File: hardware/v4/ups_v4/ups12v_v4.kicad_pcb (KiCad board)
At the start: 4 copper layers, 152 parts, among them IC1 BQ25798RQMR, J1 ADAPTER 4.75-21V, J2 VSYS OUTPUT, J3 BATTERY 2S/4S, J4 MCU / BIAS INTERFACE, J6 NTC temp sensor, J7 USB-C PROGRAM / NATIVE USB, J8 5V / GND, Q1 AON7528, Q10 AON7528, Q2 AON7528, Q3 PMV16UN, Q4 BC847 INT DOMAIN ISOLATOR, Q5 BC857 MAIN-GATED CHG SOURCE, Q6 BC847 MAIN_VALID SINK, Q7 BC847 MCU CHG ARM SINK, Q8 PMV16UN MAIN_VALID, Q9 PMV16UN TCA_EN, SW1 BOOT / DOWNLOAD, SW2 RESET, U1 ESP32-C3-MINI-1-N4X, U2 TPD2EUSB30A (PROVISIONAL), U3 TPS62933DRLR NORMAL 3V3, U4 AP7361C-33E-13 USB 3V3 LDO, U5 TPS2116DRL NORMAL PRIORITY, U6 TCA9517DGKR REV.D, U7 TPS62933DRLR, U8 LM74700QDBVRQ1

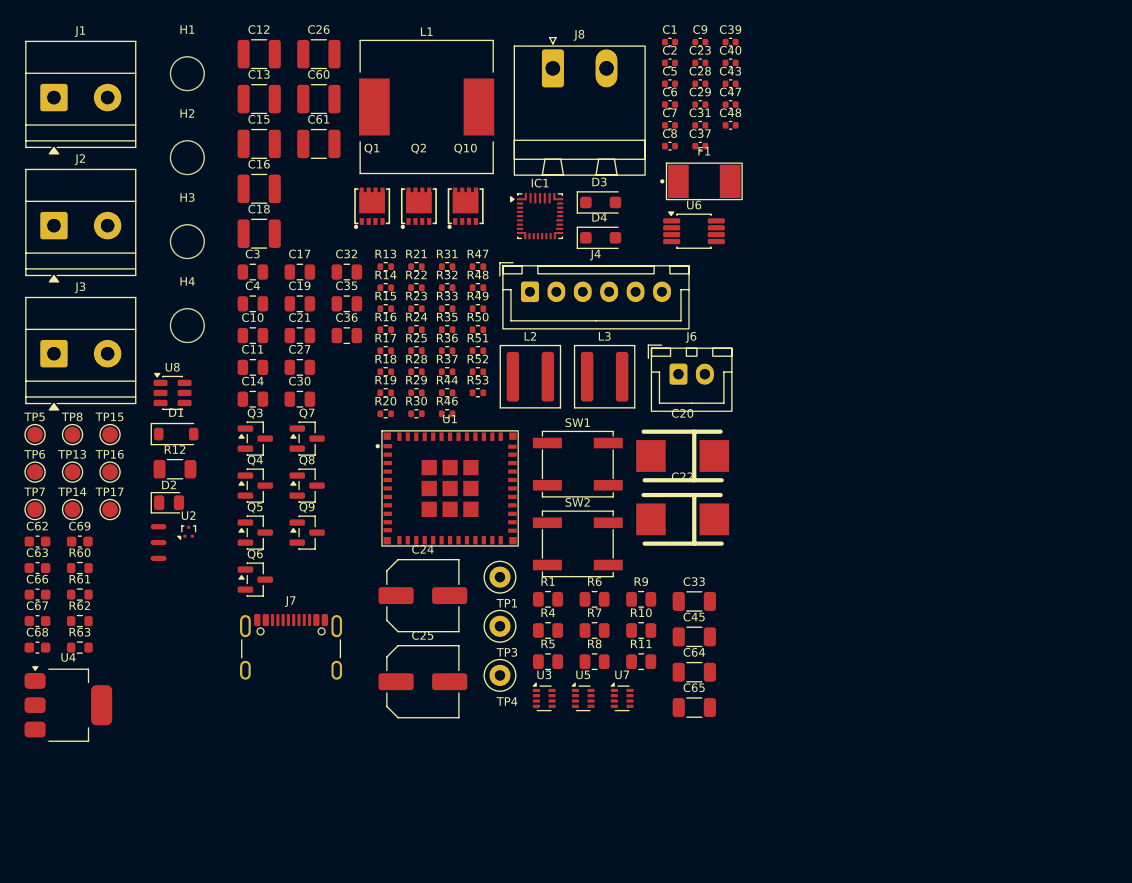
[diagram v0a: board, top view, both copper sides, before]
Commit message: phase 4.3
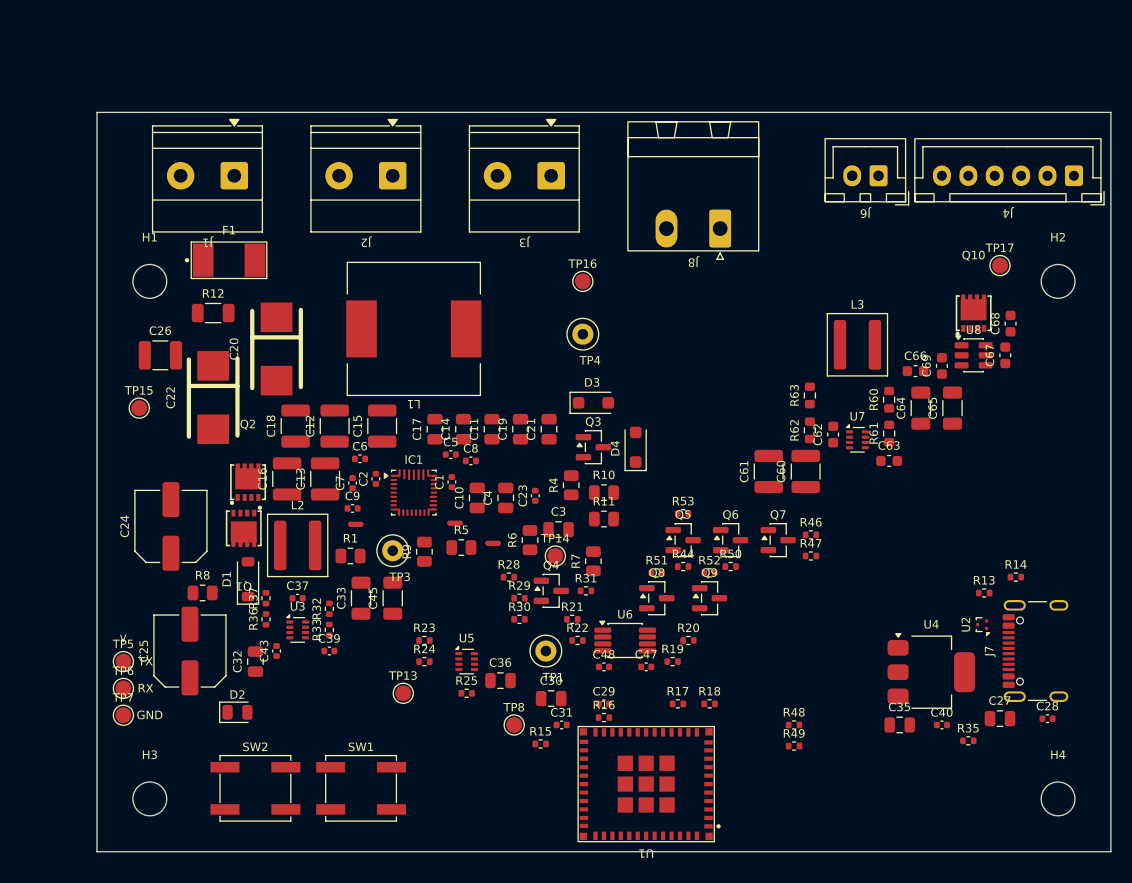
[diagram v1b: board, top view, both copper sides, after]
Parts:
- moved C68 97.1 mm to (116.5, 50.0), turned to 90 degrees
- moved C67 95.0 mm to (116.0, 53.0), turned to 90 degrees
- moved H4 93.8 mm to (121.0, 95.0)
- moved TP17 87.4 mm to (115.5, 44.5)
- moved C66 85.8 mm to (107.5, 54.5)
- moved C69 83.3 mm to (110.0, 54.0), turned to 90 degrees
- moved H2 83.3 mm to (121.0, 46.0)
- moved U4 81.8 mm to (109.0, 83.0)
- moved C63 81.3 mm to (105.0, 63.0)
- moved R60 78.3 mm to (105.0, 57.2), turned to 90 degrees
- moved R61 78.1 mm to (105.0, 60.4), turned to 90 degrees
- moved C62 76.0 mm to (99.7, 60.5), turned to 90 degrees
- moved U8 75.9 mm to (113.0, 53.0)
- moved U2 75.6 mm to (113.8, 78.5), turned to 90 degrees
- moved C27 74.2 mm to (115.5, 87.4)
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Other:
- board outline added: 96 x 70 mm
- board text added: ">"
- board text added: "GND"
- board text added: "RF: ALL LAYERS CLEAR - 15 mm EXTERNAL METAL CLEARANCE"
- board text added: "RX"
- board text added: "TX"
